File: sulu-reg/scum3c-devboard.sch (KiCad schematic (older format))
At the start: 36 parts, among them J1 Conn_02x11_Odd_Even, J2 Conn_02x10_Odd_Even, J3 Conn_02x05_Odd_Even, J4 73391-0060, U2 S-85S1AB18-I6T1U, U3 S-85S1AB11-I6T1U, U9AB1 ICM-20948

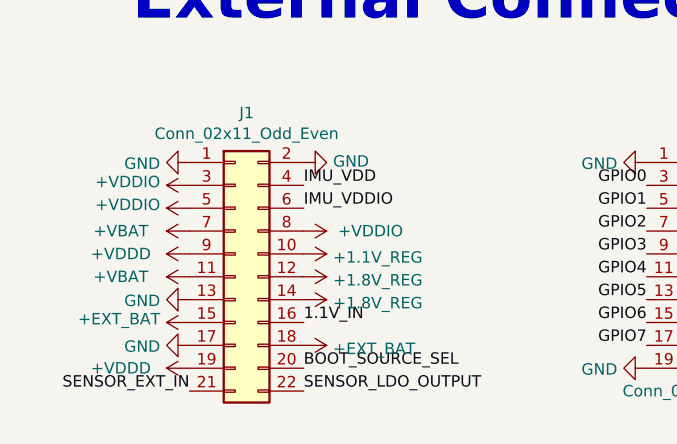
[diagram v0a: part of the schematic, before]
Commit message: rearranged some architecture
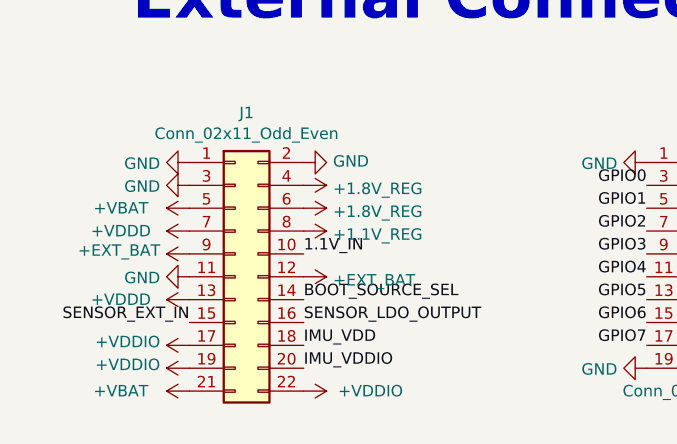
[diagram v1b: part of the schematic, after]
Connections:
- net +1.1V_REG: now also J1.8 (Pin_8); no longer J1.10 (Pin_10)
- net +1.8V_REG: now also J1.4 (Pin_4), J1.6 (Pin_6); no longer J1.12 (Pin_12), J1.14 (Pin_14)
- net +EXT_BAT: now also J1.12 (Pin_12), J1.9 (Pin_9); no longer J1.15 (Pin_15), J1.18 (Pin_18)
- net +VBAT: now also J1.21 (Pin_21), J1.5 (Pin_5); no longer J1.11 (Pin_11), J1.7 (Pin_7)
- net +VDDD: now also J1.13 (Pin_13), J1.7 (Pin_7); no longer J1.19 (Pin_19), J1.9 (Pin_9)
- net +VDDIO: now also J1.17 (Pin_17), J1.19 (Pin_19), J1.22 (Pin_22); no longer J1.3 (Pin_3), J1.5 (Pin_5), J1.8 (Pin_8)
- net 1.1V_IN: now also J1.10 (Pin_10); no longer J1.16 (Pin_16)
- net BOOT_SOURCE_SEL: now also J1.14 (Pin_14); no longer J1.20 (Pin_20)
- net GND: now also J1.11 (Pin_11), J1.3 (Pin_3); no longer J1.13 (Pin_13), J1.17 (Pin_17)
- net IMU_VDD: now also J1.18 (Pin_18); no longer J1.4 (Pin_4)
- net IMU_VDDIO: now also J1.20 (Pin_20); no longer J1.6 (Pin_6)
- net SENSOR_EXT_IN: now also J1.15 (Pin_15); no longer J1.21 (Pin_21)
- net SENSOR_LDO_OUTPUT: now also J1.16 (Pin_16); no longer J1.22 (Pin_22)
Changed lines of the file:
@@
 Text Label 1700 1750 2    50   ~ 0
 IMU_VDDIO
-Text Label 1800 7000 0    50   ~ 0
+Text Label 1800 7700 0    50   ~ 0
 IMU_VDDIO
 Text Label 3800 7300 0    50   ~ 0
@@
 Text Label 3800 7600 0    50   ~ 0
 GPIO15
-Text Label 1800 6900 0    50   ~ 0
+Text Label 1800 7600 0    50   ~ 0
 IMU_VDD
 NoConn ~ 1300 2950
@@
 	0    1    1    0
 $EndComp
-Text Label 1800 7700 0    50   ~ 0
+Text Label 1800 7400 0    50   ~ 0
 BOOT_SOURCE_SEL
 Text Label 5450 7150 0    50   ~ 0
@@
 	0    1    1    0
 $EndComp
-Text Label 1300 7800 2    50   ~ 0
-SENSOR_EXT_IN
-Text Label 1800 7800 0    50   ~ 0
+Text Label 1800 7500 0    50   ~ 0
 SENSOR_LDO_OUTPUT
 Text Label 4950 6950 2    50   ~ 0
@@
 RsTx
 $Comp
-L draft1library:+VDDIO #PWR?
-U 1 1 6076CC41
-P 1300 7000
-AR Path="/5F3B1D81/6076CC41" Ref="#PWR?"  Part="1"
-AR Path="/6076CC41" Ref="#PWR05"  Part="1"
-F 0 "#PWR05" H 1300 6850 50  0001 C CNN
-F 1 "+VDDIO" V 1315 7128 50  0000 L CNN
-F 2 "" H 1300 7000 50  0001 C CNN
-F 3 "" H 1300 7000 50  0001 C CNN
-	1    1300 7000
-	0    -1   -1   0
-$EndComp
-$Comp
-L draft1library:+VDDIO #PWR?
-U 1 1 6076D2AC
-P 1300 6900
-AR Path="/5F3B1D81/6076D2AC" Ref="#PWR?"  Part="1"
-AR Path="/6076D2AC" Ref="#PWR04"  Part="1"
-F 0 "#PWR04" H 1300 6750 50  0001 C CNN
-F 1 "+VDDIO" V 1315 7028 50  0000 L CNN
-F 2 "" H 1300 6900 50  0001 C CNN
-F 3 "" H 1300 6900 50  0001 C CNN
-	1    1300 6900
-	0    -1   -1   0
-$EndComp
-$Comp
 L draft1library:+VBAT #PWR?
 U 1 1 6076D7B9
-P 1300 7100
+P 1300 7800
 AR Path="/5F3B1D81/6076D7B9" Ref="#PWR?"  Part="1"
 AR Path="/5F41418C/6076D7B9" Ref="#PWR?"  Part="1"
 AR Path="/5F414989/6076D7B9" Ref="#PWR?"  Part="1"
 AR Path="/6076D7B9" Ref="#PWR06"  Part="1"
-F 0 "#PWR06" H 1300 6950 50  0001 C CNN
-F 1 "+VBAT" V 1300 7400 50  0000 C CNN
-F 2 "" H 1300 7100 50  0001 C CNN
-F 3 "" H 1300 7100 50  0001 C CNN
-	1    1300 7100
+F 0 "#PWR06" H 1300 7650 50  0001 C CNN
+F 1 "+VBAT" V 1300 8100 50  0000 C CNN
+F 2 "" H 1300 7800 50  0001 C CNN
+F 3 "" H 1300 7800 50  0001 C CNN
+	1    1300 7800
 	0    -1   -1   0
 $EndComp
@@
 L draft1library:+VBAT #PWR?
 U 1 1 6127ADAC
-P 1300 7300
+P 1300 7000
 AR Path="/5F3B1D81/6127ADAC" Ref="#PWR?"  Part="1"
 AR Path="/5F41418C/6127ADAC" Ref="#PWR?"  Part="1"
 AR Path="/5F414989/6127ADAC" Ref="#PWR?"  Part="1"
 AR Path="/6127ADAC" Ref="#PWR0107"  Part="1"
-F 0 "#PWR0107" H 1300 7150 50  0001 C CNN
-F 1 "+VBAT" V 1300 7600 50  0000 C CNN
-F 2 "" H 1300 7300 50  0001 C CNN
-F 3 "" H 1300 7300 50  0001 C CNN
-	1    1300 7300
+F 0 "#PWR0107" H 1300 6850 50  0001 C CNN
+F 1 "+VBAT" V 1300 7300 50  0000 C CNN
+F 2 "" H 1300 7000 50  0001 C CNN
+F 3 "" H 1300 7000 50  0001 C CNN
+	1    1300 7000
 	0    -1   -1   0
 $EndComp
@@
 L power:GND #PWR0108
 U 1 1 6127B18B
-P 1300 7400
-F 0 "#PWR0108" H 1300 7150 50  0001 C CNN
-F 1 "GND" V 1305 7272 50  0000 R CNN
-F 2 "" H 1300 7400 50  0001 C CNN
-F 3 "" H 1300 7400 50  0001 C CNN
-	1    1300 7400
-	0    1    1    0
-$EndComp
-$Comp
-L power:GND #PWR0109
-U 1 1 6127B4FF
-P 1300 7600
-F 0 "#PWR0109" H 1300 7350 50  0001 C CNN
-F 1 "GND" V 1305 7472 50  0000 R CNN
-F 2 "" H 1300 7600 50  0001 C CNN
-F 3 "" H 1300 7600 50  0001 C CNN
-	1    1300 7600
+P 1300 6900
+F 0 "#PWR0108" H 1300 6650 50  0001 C CNN
+F 1 "GND" V 1305 6772 50  0000 R CNN
+F 2 "" H 1300 6900 50  0001 C CNN
+F 3 "" H 1300 6900 50  0001 C CNN
+	1    1300 6900
 	0    1    1    0
 $EndComp
@@
 L draft1library:+1.1V_REG #PWR0110
 U 1 1 61280E78
-P 1800 7200
-F 0 "#PWR0110" H 1800 7050 50  0001 C CNN
-F 1 "+1.1V_REG" V 1815 7328 50  0000 L CNN
-F 2 "" H 1800 7200 50  0001 C CNN
-F 3 "" H 1800 7200 50  0001 C CNN
-	1    1800 7200
+P 1800 7100
+F 0 "#PWR0110" H 1800 6950 50  0001 C CNN
+F 1 "+1.1V_REG" V 1815 7228 50  0000 L CNN
+F 2 "" H 1800 7100 50  0001 C CNN
+F 3 "" H 1800 7100 50  0001 C CNN
+	1    1800 7100
 	0    1    1    0
 $EndComp
@@
 L draft1library:+1.8V_REG #PWR0111
 U 1 1 61281B91
+P 1800 6900
+F 0 "#PWR0111" H 1800 6750 50  0001 C CNN
+F 1 "+1.8V_REG" V 1815 7028 50  0000 L CNN
+F 2 "" H 1800 6900 50  0001 C CNN
+F 3 "" H 1800 6900 50  0001 C CNN
+	1    1800 6900
+	0    1    1    0
+$EndComp
+$Comp
+L draft1library:+1.8V_REG #PWR0112
+U 1 1 612829BE
+P 1800 7000
+F 0 "#PWR0112" H 1800 6850 50  0001 C CNN
+F 1 "+1.8V_REG" V 1815 7128 50  0000 L CNN
+F 2 "" H 1800 7000 50  0001 C CNN
+F 3 "" H 1800 7000 50  0001 C CNN
+	1    1800 7000
+	0    1    1    0
+$EndComp
+$Comp
+L draft1library:+EXT_BAT #PWR0113
+U 1 1 612835E6
 P 1800 7300
-F 0 "#PWR0111" H 1800 7150 50  0001 C CNN
-F 1 "+1.8V_REG" V 1815 7428 50  0000 L CNN
+F 0 "#PWR0113" H 1800 7150 50  0001 C CNN
+F 1 "+EXT_BAT" V 1815 7428 50  0000 L CNN
 F 2 "" H 1800 7300 50  0001 C CNN
 F 3 "" H 1800 7300 50  0001 C CNN
 	1    1800 7300
-	0    1    1    0
-$EndComp
-$Comp
-L draft1library:+1.8V_REG #PWR0112
-U 1 1 612829BE
-P 1800 7400
-F 0 "#PWR0112" H 1800 7250 50  0001 C CNN
-F 1 "+1.8V_REG" V 1815 7528 50  0000 L CNN
-F 2 "" H 1800 7400 50  0001 C CNN
-F 3 "" H 1800 7400 50  0001 C CNN
-	1    1800 7400
-	0    1    1    0
-$EndComp
-$Comp
-L draft1library:+EXT_BAT #PWR0113
-U 1 1 612835E6
-P 1800 7600
-F 0 "#PWR0113" H 1800 7450 50  0001 C CNN
-F 1 "+EXT_BAT" V 1815 7728 50  0000 L CNN
-F 2 "" H 1800 7600 50  0001 C CNN
-F 3 "" H 1800 7600 50  0001 C CNN
-	1    1800 7600
 	0    1    1    0
 $EndComp
@@
 L draft1library:+VDDD #PWR0125
 U 1 1 612C7D86
-P 1300 7200
-F 0 "#PWR0125" H 1300 7050 50  0001 C CNN
-F 1 "+VDDD" V 1300 7500 50  0000 C CNN
-F 2 "" H 1300 7200 50  0001 C CNN
-F 3 "" H 1300 7200 50  0001 C CNN
-	1    1300 7200
-	0    -1   -1   0
-$EndComp
-$Comp
-L draft1library:+VDDIO #PWR?
-U 1 1 6076E794
-P 1800 7100
-AR Path="/5F3B1D81/6076E794" Ref="#PWR?"  Part="1"
-AR Path="/6076E794" Ref="#PWR08"  Part="1"
-F 0 "#PWR08" H 1800 6950 50  0001 C CNN
-F 1 "+VDDIO" V 1800 7250 50  0000 L CNN
-F 2 "" H 1800 7100 50  0001 C CNN
-F 3 "" H 1800 7100 50  0001 C CNN
-	1    1800 7100
-	0    1    1    0
-$EndComp
-$Comp
-L draft1library:+VDDD #PWR07
-U 1 1 60769F1D
-P 1300 7700
-F 0 "#PWR07" H 1300 7550 50  0001 C CNN
-F 1 "+VDDD" V 1300 8000 50  0000 C CNN
-F 2 "" H 1300 7700 50  0001 C CNN
-F 3 "" H 1300 7700 50  0001 C CNN
-	1    1300 7700
+P 1300 7100
+F 0 "#PWR0125" H 1300 6950 50  0001 C CNN
+F 1 "+VDDD" V 1300 7400 50  0000 C CNN
+F 2 "" H 1300 7100 50  0001 C CNN
+F 3 "" H 1300 7100 50  0001 C CNN
+	1    1300 7100
 	0    -1   -1   0
 $EndComp
@@
 	1    0    0    -1
 $EndComp
-Text Label 1800 7500 0    50   ~ 0
+Text Label 1800 7200 0    50   ~ 0
 1.1V_IN
-$Comp
-L draft1library:+EXT_BAT #PWR0123
-U 1 1 6136676E
-P 1300 7500
-F 0 "#PWR0123" H 1300 7350 50  0001 C CNN
-F 1 "+EXT_BAT" V 1315 7628 50  0000 L CNN
-F 2 "" H 1300 7500 50  0001 C CNN
-F 3 "" H 1300 7500 50  0001 C CNN
-	1    1300 7500
-	0    -1   -1   0
-$EndComp
 Text Label 1200 5300 2    50   ~ 0
 1.1V_IN
@@
 $Comp
 L 73391-0060:73391-0060 J4
-U 1 1 613314E8
+U 1 1 61345EE5
 P 4650 2250
 F 0 "J4" H 4612 2564 50  0000 C CNN
@@
 	1    0    0    -1
 $EndComp
+$Comp
+L draft1library:+VDDIO #PWR?
+U 1 1 6076E794
+P 1800 7800
+AR Path="/5F3B1D81/6076E794" Ref="#PWR?"  Part="1"
+AR Path="/6076E794" Ref="#PWR08"  Part="1"
+F 0 "#PWR08" H 1800 7650 50  0001 C CNN
+F 1 "+VDDIO" V 1800 7950 50  0000 L CNN
+F 2 "" H 1800 7800 50  0001 C CNN
+F 3 "" H 1800 7800 50  0001 C CNN
+	1    1800 7800
+	0    1    1    0
+$EndComp
+$Comp
+L draft1library:+EXT_BAT #PWR0123
+U 1 1 6136676E
+P 1300 7200
+F 0 "#PWR0123" H 1300 7050 50  0001 C CNN
+F 1 "+EXT_BAT" V 1315 7328 50  0000 L CNN
+F 2 "" H 1300 7200 50  0001 C CNN
+F 3 "" H 1300 7200 50  0001 C CNN
+	1    1300 7200
+	0    -1   -1   0
+$EndComp
+$Comp
+L draft1library:+VDDD #PWR07
+U 1 1 60769F1D
+P 1300 7400
+F 0 "#PWR07" H 1300 7250 50  0001 C CNN
+F 1 "+VDDD" V 1300 7700 50  0000 C CNN
+F 2 "" H 1300 7400 50  0001 C CNN
+F 3 "" H 1300 7400 50  0001 C CNN
+	1    1300 7400
+	0    -1   -1   0
+$EndComp
+$Comp
+L power:GND #PWR0109
+U 1 1 6127B4FF
+P 1300 7300
+F 0 "#PWR0109" H 1300 7050 50  0001 C CNN
+F 1 "GND" V 1305 7172 50  0000 R CNN
+F 2 "" H 1300 7300 50  0001 C CNN
+F 3 "" H 1300 7300 50  0001 C CNN
+	1    1300 7300
+	0    1    1    0
+$EndComp
+$Comp
+L draft1library:+VDDIO #PWR?
+U 1 1 6076D2AC
+P 1300 7600
+AR Path="/5F3B1D81/6076D2AC" Ref="#PWR?"  Part="1"
+AR Path="/6076D2AC" Ref="#PWR04"  Part="1"
+F 0 "#PWR04" H 1300 7450 50  0001 C CNN
+F 1 "+VDDIO" V 1315 7728 50  0000 L CNN
+F 2 "" H 1300 7600 50  0001 C CNN
+F 3 "" H 1300 7600 50  0001 C CNN
+	1    1300 7600
+	0    -1   -1   0
+$EndComp
+$Comp
+L draft1library:+VDDIO #PWR?
+U 1 1 6076CC41
+P 1300 7700
+AR Path="/5F3B1D81/6076CC41" Ref="#PWR?"  Part="1"
+AR Path="/6076CC41" Ref="#PWR05"  Part="1"
+F 0 "#PWR05" H 1300 7550 50  0001 C CNN
+F 1 "+VDDIO" V 1315 7828 50  0000 L CNN
+F 2 "" H 1300 7700 50  0001 C CNN
+F 3 "" H 1300 7700 50  0001 C CNN
+	1    1300 7700
+	0    -1   -1   0
+$EndComp
+Text Label 1300 7500 2    50   ~ 0
+SENSOR_EXT_IN
 $EndSCHEMATC
